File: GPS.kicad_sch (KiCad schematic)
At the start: 16 parts, among them J11 GPS_I2C, J12 GPS_BAT, SW4 GPS_RESET, U9 PA1616S_GPS

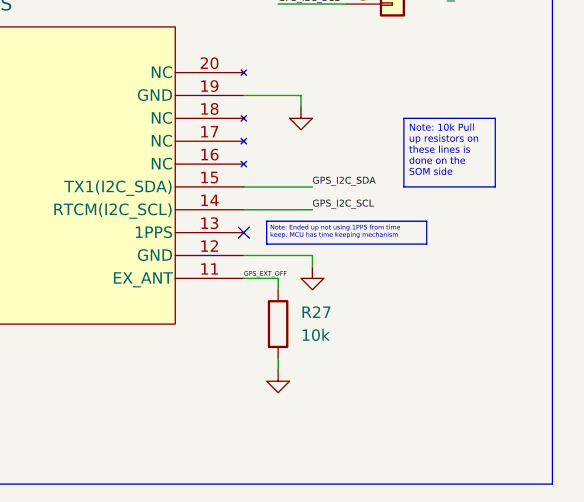
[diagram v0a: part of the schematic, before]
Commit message: fix errors schem
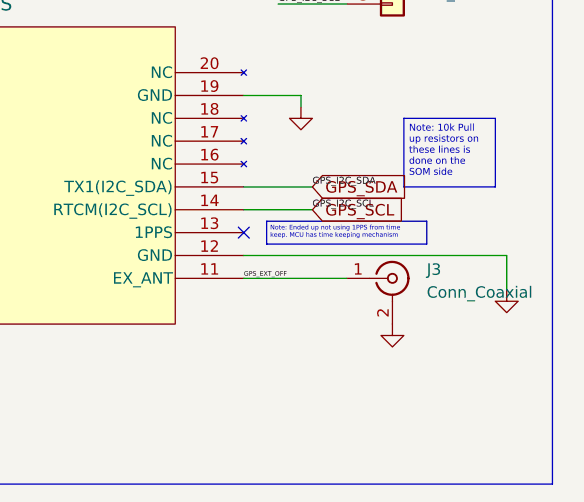
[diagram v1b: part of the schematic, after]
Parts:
- removed R27: 10k, Resistor_SMD:R_0805_2012Metric, symbol Device:R
- added J3: Conn_Coaxial, symbol Connector:Conn_Coaxial
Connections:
- net GND: now also J3.2 (Ext)
- net GPS_EXT_OFF: now also J3.1 (In)
- net GPS_I2C_SCL renamed GPS_SCL
- net GPS_I2C_SDA renamed GPS_SDA
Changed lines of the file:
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@@
 	(wire
 		(pts
-			(xy 190.5 113.03) (xy 198.12 113.03)
+			(xy 190.5 113.03) (xy 219.71 113.03)
 		)
 		(stroke
@@
 	(wire
 		(pts
-			(xy 198.12 113.03) (xy 198.12 114.3)
+			(xy 219.71 113.03) (xy 219.71 116.84)
 		)
 		(stroke
@@
 	(wire
 		(pts
-			(xy 194.31 124.46) (xy 194.31 125.73)
-		)
-		(stroke
-			(width 0)
-			(type default)
-		)
-	)
-	(wire
-		(pts
 			(xy 78.74 106.68) (xy 78.74 104.14)
 		)
@@
 	(wire
 		(pts
-			(xy 194.31 116.84) (xy 194.31 115.57)
-		)
-		(stroke
-			(width 0)
-			(type default)
-		)
-	)
-	(wire
-		(pts
 			(xy 194.31 82.55) (xy 201.93 82.55)
 		)
@@
 	(wire
 		(pts
-			(xy 194.31 115.57) (xy 190.5 115.57)
+			(xy 190.5 115.57) (xy 201.93 115.57)
 		)
 		(stroke
@@
 		)
 	)
+	(global_label "GPS_SCL"
+		(shape input)
+		(at 198.12 107.95 0)
+		(fields_autoplaced yes)
+		(effects
+			(font
+				(size 1.27 1.27)
+			)
+			(justify left)
+		)
+		(property "Intersheetrefs" "${INTERSHEET_REFS}"
+			(at 209.3299 107.95 0)
+			(effects
+				(font
+					(size 1.27 1.27)
+				)
+				(justify left)
+				(hide yes)
+			)
+		)
+	)
+	(global_label "GPS_SDA"
+		(shape input)
+		(at 198.12 105.41 0)
+		(fields_autoplaced yes)
+		(effects
+			(font
+				(size 1.27 1.27)
+			)
+			(justify left)
+		)
+		(property "Intersheetrefs" "${INTERSHEET_REFS}"
+			(at 209.3904 105.41 0)
+			(effects
+				(font
+					(size 1.27 1.27)
+				)
+				(justify left)
+				(hide yes)
+			)
+		)
+	)
 	(symbol
 		(lib_id "power:PWR_FLAG")
@@
 	(symbol
 		(lib_id "power:GND")
-		(at 194.31 125.73 0)
-		(unit 1)
-		(exclude_from_sim no)
-		(in_bom yes)
-		(on_board yes)
-		(dnp no)
-		(fields_autoplaced yes)
-		(property "Reference" "#PWR078"
-			(at 194.31 132.08 0)
-			(effects
-				(font
-					(size 1.27 1.27)
-				)
-				(hide yes)
-			)
-		)
-		(property "Value" "GND"
-			(at 194.31 130.81 0)
-			(effects
-				(font
-					(size 1.27 1.27)
-				)
-				(hide yes)
-			)
-		)
-		(property "Footprint" ""
-			(at 194.31 125.73 0)
-			(effects
-				(font
-					(size 1.27 1.27)
-				)
-				(hide yes)
-			)
-		)
-		(property "Datasheet" ""
-			(at 194.31 125.73 0)
-			(effects
-				(font
-					(size 1.27 1.27)
-				)
-				(hide yes)
-			)
-		)
-		(property "Description" "Power symbol creates a global label with name \"GND\" , ground"
-			(at 194.31 125.73 0)
-			(effects
-				(font
-					(size 1.27 1.27)
-				)
-				(hide yes)
-			)
-		)
-		(pin "1"
-		)
-		(instances
-			(project "TSOMProject"
-				(path "/f13eb969-5de0-437e-a1b7-e0204111e0b2/d8680ae9-0acb-42e1-892b-ebdc48294ea6"
-					(reference "#PWR078")
-					(unit 1)
-				)
-			)
-		)
-	)
-	(symbol
-		(lib_id "power:GND")
 		(at 101.6 73.66 0)
 		(unit 1)
@@
 	)
 	(symbol
+		(lib_id "Connector:Conn_Coaxial")
+		(at 207.01 115.57 0)
+		(unit 1)
+		(exclude_from_sim no)
+		(in_bom yes)
+		(on_board yes)
+		(dnp no)
+		(property "Reference" "J3"
+			(at 210.82 114.5931 0)
+			(effects
+				(font
+					(size 1.27 1.27)
+				)
+				(justify left)
+			)
+		)
+		(property "Value" "Conn_Coaxial"
+			(at 210.82 117.1331 0)
+			(effects
+				(font
+					(size 1.27 1.27)
+				)
+				(justify left)
+			)
+		)
+		(property "Footprint" ""
+			(at 207.01 115.57 0)
+			(effects
+				(font
+					(size 1.27 1.27)
+				)
+				(hide yes)
+			)
+		)
+		(property "Datasheet" "~"
+			(at 207.01 115.57 0)
+			(effects
+				(font
+					(size 1.27 1.27)
+				)
+				(hide yes)
+			)
+		)
+		(property "Description" "coaxial connector (BNC, SMA, SMB, SMC, Cinch/RCA, LEMO, ...)"
+			(at 207.01 115.57 0)
+			(effects
+				(font
+					(size 1.27 1.27)
+				)
+				(hide yes)
+			)
+		)
+		(pin "1"
+		)
+		(pin "2"
+		)
+		(instances
+			(project ""
+				(path "/f13eb969-5de0-437e-a1b7-e0204111e0b2/d8680ae9-0acb-42e1-892b-ebdc48294ea6"
+					(reference "J3")
+					(unit 1)
+				)
+			)
+		)
+	)
+	(symbol
 		(lib_id "Switch:SW_Push")
 		(at 83.82 88.9 0)
@@
 	)
 	(symbol
+		(lib_id "power:GND")
+		(at 207.01 120.65 0)
+		(unit 1)
+		(exclude_from_sim no)
+		(in_bom yes)
+		(on_board yes)
+		(dnp no)
+		(fields_autoplaced yes)
+		(property "Reference" "#PWR041"
+			(at 207.01 127 0)
+			(effects
+				(font
+					(size 1.27 1.27)
+				)
+				(hide yes)
+			)
+		)
+		(property "Value" "GND"
+			(at 207.01 125.73 0)
+			(effects
+				(font
+					(size 1.27 1.27)
+				)
+				(hide yes)
+			)
+		)
+		(property "Footprint" ""
+			(at 207.01 120.65 0)
+			(effects
+				(font
+					(size 1.27 1.27)
+				)
+				(hide yes)
+			)
+		)
+		(property "Datasheet" ""
+			(at 207.01 120.65 0)
+			(effects
+				(font
+					(size 1.27 1.27)
+				)
+				(hide yes)
+			)
+		)
+		(property "Description" "Power symbol creates a global label with name \"GND\" , ground"
+			(at 207.01 120.65 0)
+			(effects
+				(font
+					(size 1.27 1.27)
+				)
+				(hide yes)
+			)
+		)
+		(pin "1"
+		)
+		(instances
+			(project "TSOMProject"
+				(path "/f13eb969-5de0-437e-a1b7-e0204111e0b2/d8680ae9-0acb-42e1-892b-ebdc48294ea6"
+					(reference "#PWR041")
+					(unit 1)
+				)
+			)
+		)
+	)
+	(symbol
 		(lib_id "Connector_Generic:Conn_01x03")
 		(at 207.01 82.55 0)
@@
 	)
 	(symbol
-		(lib_id "Device:R")
-		(at 194.31 120.65 0)
-		(unit 1)
-		(exclude_from_sim no)
-		(in_bom yes)
-		(on_board yes)
-		(dnp no)
-		(fields_autoplaced yes)
-		(property "Reference" "R27"
-			(at 196.85 119.3799 0)
-			(effects
-				(font
-					(size 1.27 1.27)
-				)
-				(justify left)
-			)
-		)
-		(property "Value" "10k"
-			(at 196.85 121.9199 0)
-			(effects
-				(font
-					(size 1.27 1.27)
-				)
-				(justify left)
-			)
-		)
-		(property "Footprint" "Resistor_SMD:R_0805_2012Metric"
-			(at 192.532 120.65 90)
-			(effects
-				(font
-					(size 1.27 1.27)
-				)
-				(hide yes)
-			)
-		)
-		(property "Datasheet" "~"
-			(at 194.31 120.65 0)
-			(effects
-				(font
-					(size 1.27 1.27)
-				)
-				(hide yes)
-			)
-		)
-		(property "Description" "NRSET Pull Up"
-			(at 194.31 120.65 0)
-			(effects
-				(font
-					(size 1.27 1.27)
-				)
-				(hide yes)
-			)
-		)
-		(property "Mouser Part Number" "71-CRCW0805-10K-E3"
-			(at 194.31 120.65 0)
-			(effects
-				(font
-					(size 1.27 1.27)
-				)
-				(hide yes)
-			)
-		)
-		(property "Link" "https://www.mouser.com/ProductDetail/Vishay-Dale/CRCW080510K0FKEA?qs=LOX6nxTstiZjDFtI%2F0c8Lw%3D%3D&utm_id=8791529225&gad_source=1&gclid=CjwKCAiAhP67BhAVEiwA2E_9gwE6c5uIXF_e8E4XWu9TqUsCdxHoT8O-di25N1pJkLQVdtDpVs-qwxoCB3sQAvD_BwE"
-			(at 194.31 120.65 0)
-			(effects
-				(font
-					(size 1.27 1.27)
-				)
-				(hide yes)
-			)
-		)
-		(property "P/N" "CRCW080510K0FKEA"
-			(at 194.31 120.65 0)
-			(effects
-				(font
-					(size 1.27 1.27)
-				)
-				(hide yes)
-			)
-		)
-		(pin "1"
-		)
-		(pin "2"
-		)
-		(instances
-			(project "TSOMProject"
-				(path "/f13eb969-5de0-437e-a1b7-e0204111e0b2/d8680ae9-0acb-42e1-892b-ebdc48294ea6"
-					(reference "R27")
-					(unit 1)
-				)
-			)
-		)
-	)
-	(symbol
 		(lib_id "DataAcqLeaderBoard-Symbols:2994TR")
 		(at 80.01 116.84 90)
@@
 	(symbol
 		(lib_id "power:GND")
-		(at 198.12 114.3 0)
+		(at 219.71 116.84 0)
 		(unit 1)
 		(exclude_from_sim no)
@@
 		(fields_autoplaced yes)
 		(property "Reference" "#PWR080"
-			(at 198.12 120.65 0)
+			(at 219.71 123.19 0)
 			(effects
 				(font
@@
 		)
 		(property "Value" "GND"
-			(at 198.12 119.38 0)
+			(at 219.71 121.92 0)
 			(effects
 				(font
@@
 		)
 		(property "Footprint" ""
-			(at 198.12 114.3 0)
+			(at 219.71 116.84 0)
 			(effects
 				(font
@@
 		)
 		(property "Datasheet" ""
-			(at 198.12 114.3 0)
+			(at 219.71 116.84 0)
 			(effects
 				(font
@@
 		)
 		(property "Description" "Power symbol creates a global label with name \"GND\" , ground"
-			(at 198.12 114.3 0)
-			(effects
-				(font
+			(at 219.71 116.84 0)
+			(effects
+				(font
